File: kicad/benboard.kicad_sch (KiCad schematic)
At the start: 58 parts, among them J1 USB_C_Receptacle_USB2.0, SW1 SW_Push, U1 nRF52840, U2 BQ24075RGT, Y1 32MHz, Y2 32.768kHz

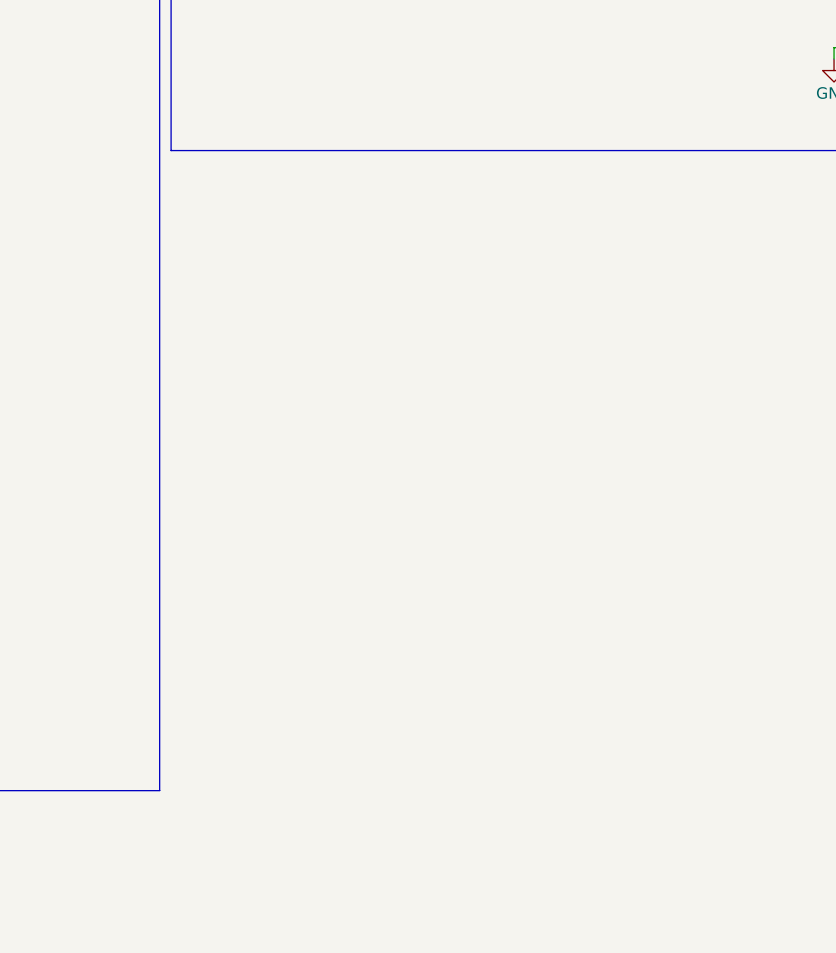
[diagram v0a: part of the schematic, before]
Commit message: more cad files as well as readme
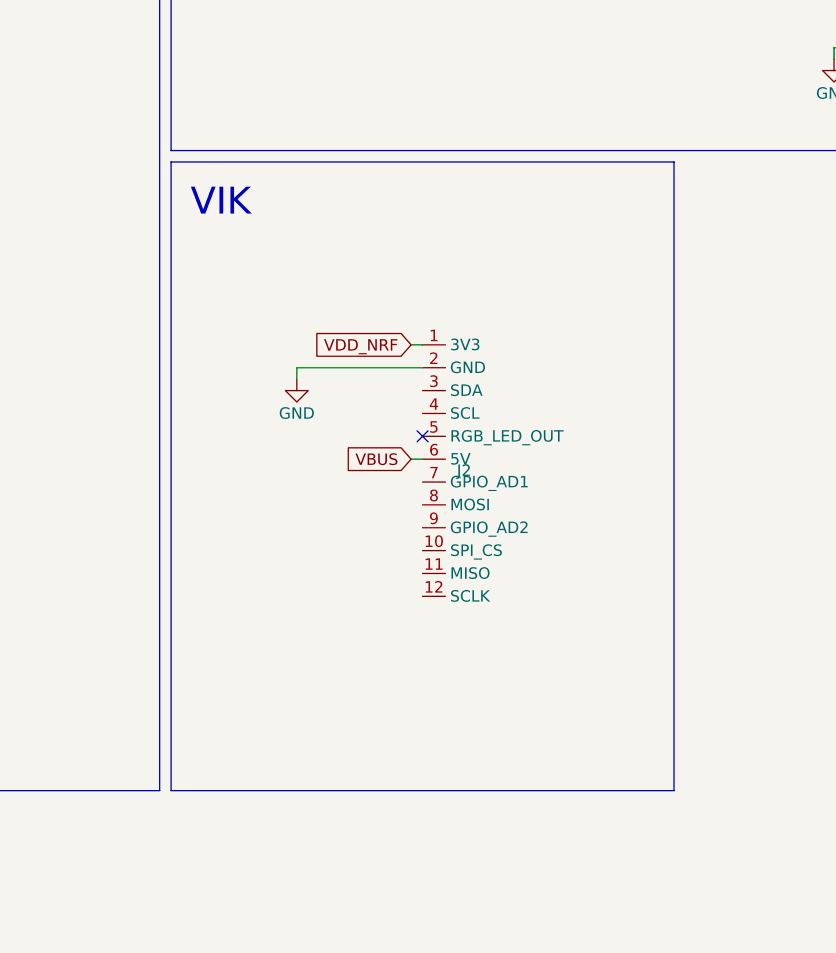
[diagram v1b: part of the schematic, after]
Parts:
- added J2: ~, symbol vik:vik-keyboard-connector
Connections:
- net GND: now also J2.2 (GND)
- net VBUS: now also J2.6 (5V)
- net VDD_NRF: now also J2.1 (3V3)
- no-connect marks 6 -> 7
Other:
- note added: "VIK"
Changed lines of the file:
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@@
   (no_connect (at 270.51 73.66))
   (no_connect (at 64.77 77.47))
+  (no_connect (at 177.8 190.5))
   (no_connect (at 171.45 62.23))
   (wire (pts (xy 116.84 181.61) (xy 115.57 181.61))
@@
     (stroke (width 0) (type default))
   )
+  (wire (pts (xy 177.8 182.88) (xy 163.83 182.88))
+    (stroke (width 0) (type default))
+  )
   (wire (pts (xy 116.84 176.53) (xy 115.57 176.53))
     (stroke (width 0) (type default))
@@
     (stroke (width 0) (type default))
   )
+  (wire (pts (xy 176.53 193.04) (xy 177.8 193.04))
+    (stroke (width 0) (type default))
+  )
   (wire (pts (xy 224.79 147.32) (xy 223.52 147.32))
     (stroke (width 0) (type default))
@@
     (stroke (width 0) (type default))
   )
+  (wire (pts (xy 176.53 180.34) (xy 177.8 180.34))
+    (stroke (width 0) (type default))
+  )
   (wire (pts (xy 100.33 35.56) (xy 100.33 36.83))
     (stroke (width 0) (type default))
@@
     (stroke (width 0) (type default))
   )
+  (wire (pts (xy 163.83 182.88) (xy 163.83 184.15))
+    (stroke (width 0) (type default))
+  )
   (wire (pts (xy 271.78 62.23) (xy 271.78 63.5))
     (stroke (width 0) (type default))
@@
   )
   (rectangle (start 149.86 12.7) (end 236.22 93.98)
+    (stroke (width 0) (type default))
+    (fill (type none))
+  )
+  (rectangle (start 149.86 160.02) (end 205.74 229.87)
     (stroke (width 0) (type default))
     (fill (type none))
@@
   )
   (text "Battery Charging\n" (at 189.23 17.78 0)
+    (effects (font (size 3 3)) (justify right bottom))
+  )
+  (text "VIK" (at 158.75 166.37 0)
     (effects (font (size 3 3)) (justify right bottom))
   )
@@
     )
   )
+  (global_label "VDD_NRF" (shape input) (at 176.53 180.34 180) (fields_autoplaced)
+    (effects (font (size 1.27 1.27)) (justify right))
+    (property "Intersheetrefs" "${INTERSHEET_REFS}" (at 165.2595 180.34 0)
+      (effects (font (size 1.27 1.27)) (justify right) hide)
+    )
+  )
   (global_label "SW20" (shape input) (at 116.84 173.99 0) (fields_autoplaced)
     (effects (font (size 1.27 1.27)) (justify left))
@@
     )
   )
+  (global_label "VBUS" (shape input) (at 176.53 193.04 180) (fields_autoplaced)
+    (effects (font (size 1.27 1.27)) (justify right))
+    (property "Intersheetrefs" "${INTERSHEET_REFS}" (at 168.6462 193.04 0)
+      (effects (font (size 1.27 1.27)) (justify right) hide)
+    )
+  )
   (global_label "VDD_NRF" (shape input) (at 82.55 53.34 90) (fields_autoplaced)
     (effects (font (size 1.27 1.27)) (justify left))
@@
         (path "/b2065370-6f3a-4205-b26a-a9c2368077cd"
           (reference "SW4") (unit 1)
+        )
+      )
+    )
+  )
+  (symbol (lib_id "vik:vik-keyboard-connector") (at 177.8 194.31 0) (unit 1)
+    (in_bom yes) (on_board yes) (dnp no) (fields_autoplaced)
+    (property "Reference" "J2" (at 181.61 194.31 0)
+      (effects (font (size 1.27 1.27)) (justify left))
+    )
+    (property "Value" "~" (at 177.8 187.96 0)
+      (effects (font (size 1.27 1.27)))
+    )
+    (property "Footprint" "" (at 177.8 187.96 0)
+      (effects (font (size 1.27 1.27)) hide)
+    )
+    (property "Datasheet" "" (at 177.8 187.96 0)
+      (effects (font (size 1.27 1.27)) hide)
+    )
+    (pin "1")
+    (pin "10")
+    (pin "11")
+    (pin "12")
+    (pin "2")
+    (pin "3")
+    (pin "4")
+    (pin "5")
+    (pin "6")
+    (pin "7")
+    (pin "8")
+    (pin "9")
+    (instances
+      (project "benboard"
+        (path "/b2065370-6f3a-4205-b26a-a9c2368077cd"
+          (reference "J2") (unit 1)
         )
       )
@@
         )
       )
+    )
+  )
+  (symbol (lib_id "power:GND") (at 163.83 184.15 0) (unit 1)
+    (in_bom yes) (on_board yes) (dnp no)
+    (property "Reference" "#PWR045" (at 163.83 190.5 0)
+      (effects (font (size 1.27 1.27)) hide)
+    )
+    (property "Value" "GND" (at 163.83 187.96 0)
+      (effects (font (size 1.27 1.27)))
+    )
+    (property "Footprint" "" (at 163.83 184.15 0)
+      (effects (font (size 1.27 1.27)) hide)
+    )
+    (property "Datasheet" "" (at 163.83 184.15 0)
+      (effects (font (size 1.27 1.27)) hide)
+    )
+    (pin "1")
+    (instances
+      (project "benboard"
+        (path "/b2065370-6f3a-4205-b26a-a9c2368077cd"
+          (reference "#PWR045") (unit 1)
+        )
+      )

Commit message: add vik
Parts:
- C1: footprint Capacitor_SMD:C_0603_1608Metric -> Connector_FFC-FPC:TE_1-84953-2_1x12-1MP_P1.0mm_Horizontal
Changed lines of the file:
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@@
       (effects (font (size 1.27 1.27)))
     )
-    (property "Footprint" "Capacitor_SMD:C_0603_1608Metric" (at 99.06 34.5948 0)
+    (property "Footprint" "Connector_FFC-FPC:TE_1-84953-2_1x12-1MP_P1.0mm_Horizontal" (at 99.06 34.5948 0)
       (effects (font (size 1.27 1.27)) hide)
     )
